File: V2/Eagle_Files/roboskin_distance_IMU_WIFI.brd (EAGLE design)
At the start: 43.2 x 33 mm, 54 parts, among them IC1 CP2104, Q1 mmbt2222, Q2 mmbt2222, SW2 KMR2, U1 LIS3DHTR, U2 AP2112-3.3, U3 MCP, U5 VL53L1XSMD, X1 JSTPH, X2 ESP-12, X4 20329

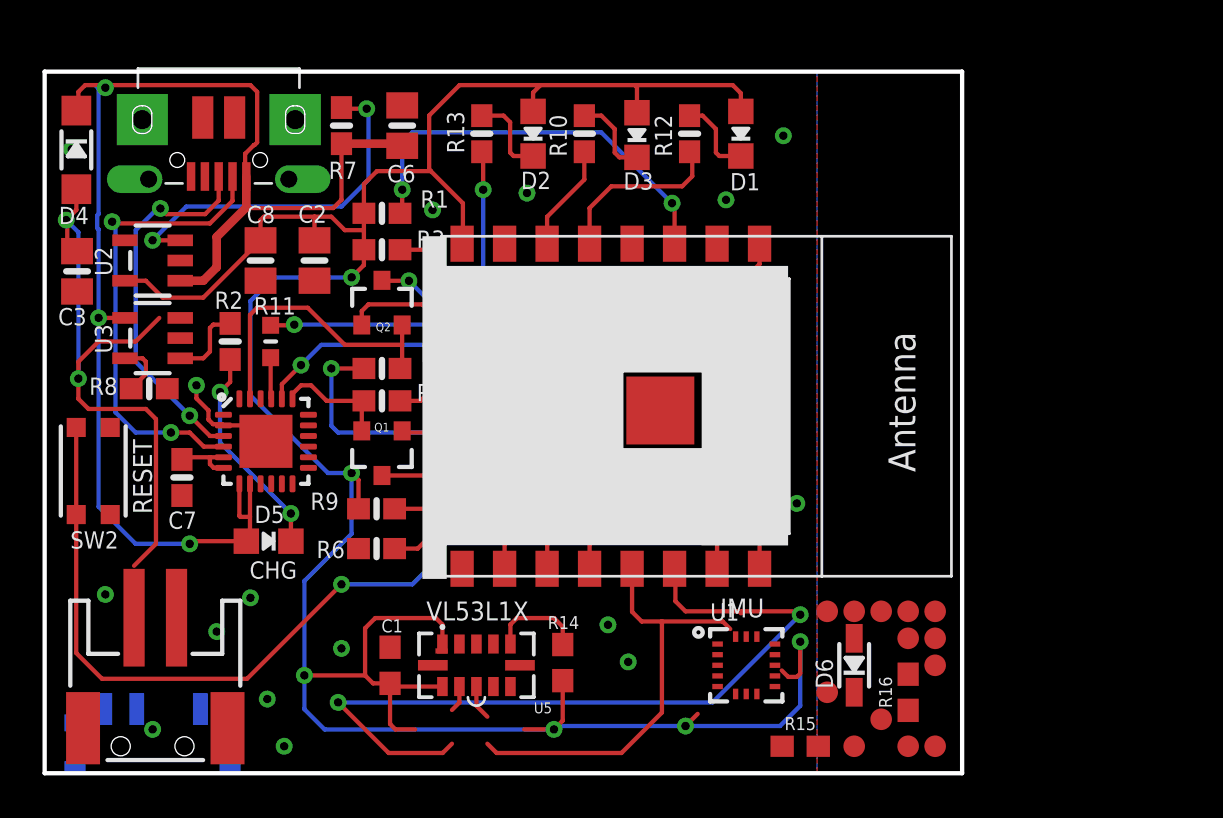
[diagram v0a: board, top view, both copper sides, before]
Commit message: All versions of hardware
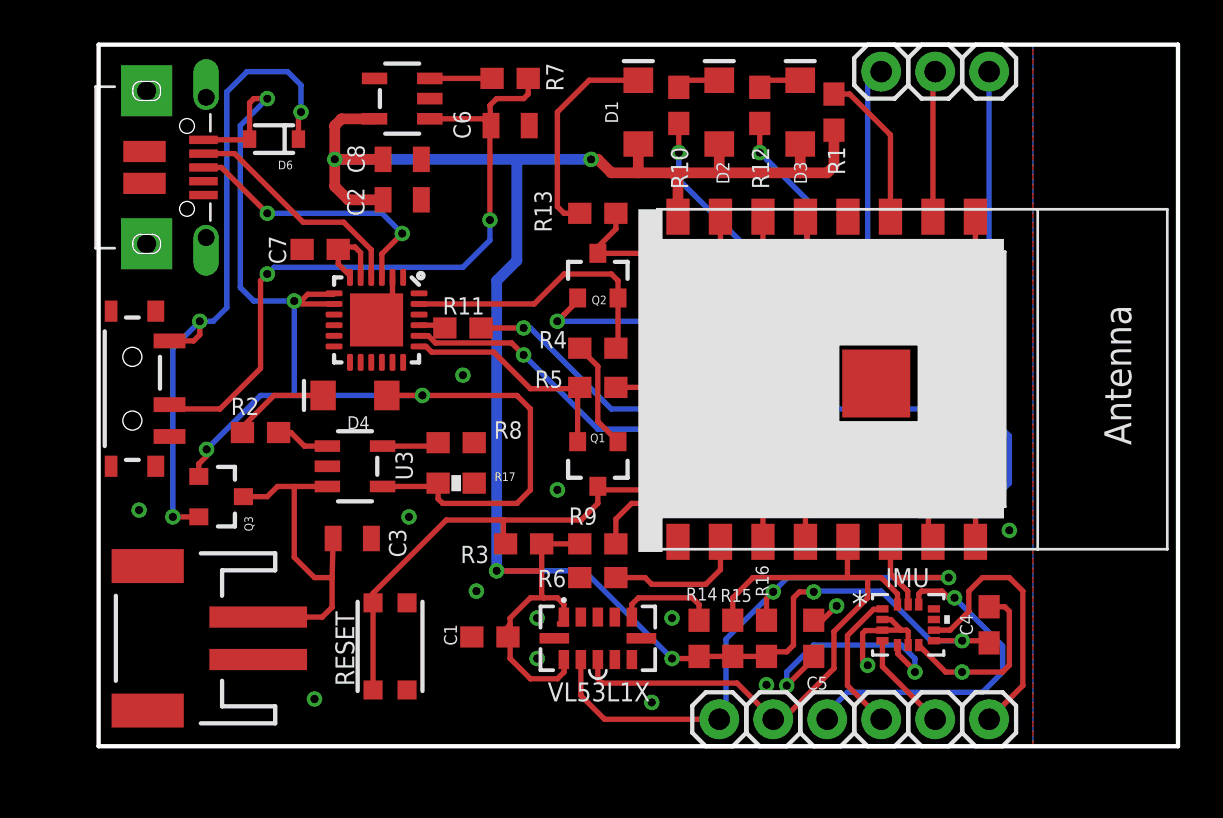
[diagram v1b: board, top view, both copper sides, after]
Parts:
- removed D5: CHG, microbuilder:CHIPLED_0805_NOOUTLINE
- removed S1: (no value), SparkFun-Switches:SWITCH_SPST_SMD_A
- removed TP1, TP10, TP11, TP12, TP13, TP2, TP3, TP4, TP5, TP6, TP7, TP8, TP9: TEST-POINT3X4, SparkFun-Connectors:PAD.03X.04
- removed X1: JSTPH, microbuilder:JSTPH2
- added C4, C5: 0.1uF, SparkFun-Capacitors:0603
- added J1, J10, J2, J3, J4, J6, J7, J8, J9: (no value), SparkFun-Connectors:1X01
- added J5: (no value), SparkFun-Connectors:JST-2-SMD
- added Q3: ZXMP6A13FTA, SparkFun-DiscreteSemi:SOT23-3
- added R17: 100k, SparkFun-Resistors:0603-RES
- added S2: POWER, SparkFun-Electromechanical:SWITCH-SPST-SMD-A
- C2: device microbuilder:0805-NO -> SparkFun-Capacitors:0805
- C3, C6, C8: value 10µF -> 10uF; device microbuilder:0805-NO -> SparkFun-Capacitors:0805
- C7: value 1uF -> 1.0uF; device microbuilder:0603-NO -> SparkFun-Capacitors:0603
- D1, D2, D3: value RED -> WHITE; device microbuilder:CHIPLED_0805_NOOUTLINE -> SparkFun-LED:LED-1206
- D4: value MBR120 -> WHITE; device microbuilder:SOD-123 -> SparkFun-LED:LED-1206
- D6: value 1N4148 -> BAT20J; device microbuilder:SOD-323 -> SparkFun-DiscreteSemi:SOD-323
- R1, R3, R4, R5, R7, R9: value 10K -> 10k; device microbuilder:0603-NO -> SparkFun-Resistors:0603
- R10, R12, R13, R2, R8: value 1K -> 1k; device microbuilder:0603-NO -> SparkFun-Resistors:0603
- R11: value 1K -> 1k; device microbuilder:_0603MP -> SparkFun-Resistors:0603
- R15, R16: value 10k -> 4.7k
- R6: value 4.7K -> 4.7k; device microbuilder:0603-NO -> SparkFun-Resistors:0603
- U1: value LIS3DHTR -> ISM330DLCTR; device microbuilder:LGA16_3X3MM -> ISM330:LGA-14L_2P5X3X0P83_STM
- moved D6 36.9 mm to (10.8, 29.8), turned to 180 degrees
- moved R1 21.8 mm to (37.1, 31.1), turned to 270 degrees
- moved C3 18.1 mm to (14.5, 11.0), turned to 0 degrees
- moved D4 17.5 mm to (14.6, 17.8), turned to 180 degrees
- moved SW2 16.2 mm to (16.3, 5.97)
- moved R3 15.4 mm to (22.5, 10.8), turned to 0 degrees
- moved R8 14.7 mm to (19.4, 15.6)
- moved U2 14.0 mm to (16.8, 31.8)
- moved C7 12.6 mm to (13.0, 24.7), turned to 180 degrees
- moved U3 11.3 mm to (14.6, 14.4), turned to 270 degrees
- moved R9 10.5 mm to (26.0, 10.8)
- moved R6 10.5 mm to (26.0, 9.21)
- moved U$6 10.2 mm to (32.1, 18.4)
- moved Q2 10.2 mm to (26.0, 23.4)
- moved X2 10.2 mm to (38.0, 18.5)
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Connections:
- removed net N$10: D2.C, R13.2
- removed net SDO: R16.2, U1.7
- removed net VBAT: D4.A, S1.2
- removed net V_CHARGE: C3.1, S1.3, U3.3, X1.2
- new net INMOSFET: D6.C, Q3.2, S2.3
- new net INT1: J3.1, U1.4
- new net INT2: J2.1, U1.9
- new net LIPO: C3.1, J5.2, Q3.3, U3.3
- new net SDAO: J1.1, U1.1
- new net VDIO: C5.1, U1.5
- new net VINPUT: C6.1, R7.2, S2.2, U2.1
- net 3.3V: now also C4.1, R15.2, R16.2, U1.8; no longer R15.1, U1.1, U1.14, U1.15
- net ADC: now also J6.1
- net CS: now also J4.1, U1.12; no longer D6.C
- net GND: now also C4.2, C5.2, J5.1, R17.1, U1.2, U1.3, U1.6, U1.7; no longer R16.1, U1.10, U1.12, U1.13, U1.16, U1.5, X1.1
- net GPIO13/MOSI: now also J8.1
- net GPIO14: now also J7.1
- net N$1: now also D4.C; no longer D5.C
- net N$5: now also D1.C, R13.2; no longer D3.C, R10.2
- net N$7: now also D2.C, R10.2; no longer D6.A, R15.2, U1.8
- net N$9: now also D3.C; no longer D1.C
- net SCL: now also J9.1, R16.1, U1.13; no longer U1.4
- net SDA: now also J10.1, R15.1, U1.14; no longer U1.6
- net VBUS: now also D4.A, D6.A, Q3.1, R17.2; no longer C6.1, D4.C, D5.A, R7.2, U2.1
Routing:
- net VINPUT: track 0.00 -> 33.0 mm, vias 0 -> 2
- net INMOSFET: track 0.00 -> 31.6 mm, vias 0 -> 3
- net VBAT: track 28.2 -> 0.00 mm, vias 2 -> 0
- net 3.3V: track 130.0 -> 107.5 mm
- net GPIO14: track 8.33 -> 29.1 mm, vias 0 -> 2
- net GPIO13/MOSI: track 0.00 -> 19.3 mm, vias 0 -> 1
- net RESET: track 65.9 -> 47.4 mm, vias 2 -> 0
- net LIPO: track 0.00 -> 16.6 mm
- net CS: track 0.00 -> 16.2 mm, vias 0 -> 1
- net EN: track 17.2 -> 2.93 mm, vias 2 -> 0
- net GND: track 4.97 -> 17.7 mm, vias 22 -> 18
- net INT2: track 0.00 -> 12.7 mm
- net CH_PD: track 19.6 -> 7.31 mm, vias 2 -> 0
- net VDIO: track 0.00 -> 11.6 mm, vias 0 -> 2
- net N$6: track 22.1 -> 11.1 mm, vias 2 -> 0
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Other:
- board size 43.2 x 33 mm -> 50.8 x 33 mm
